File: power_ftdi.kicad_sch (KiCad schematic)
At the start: 2 parts, among them J3 USB_C_Receptacle_USB2.0_14P, U3 FT4232H

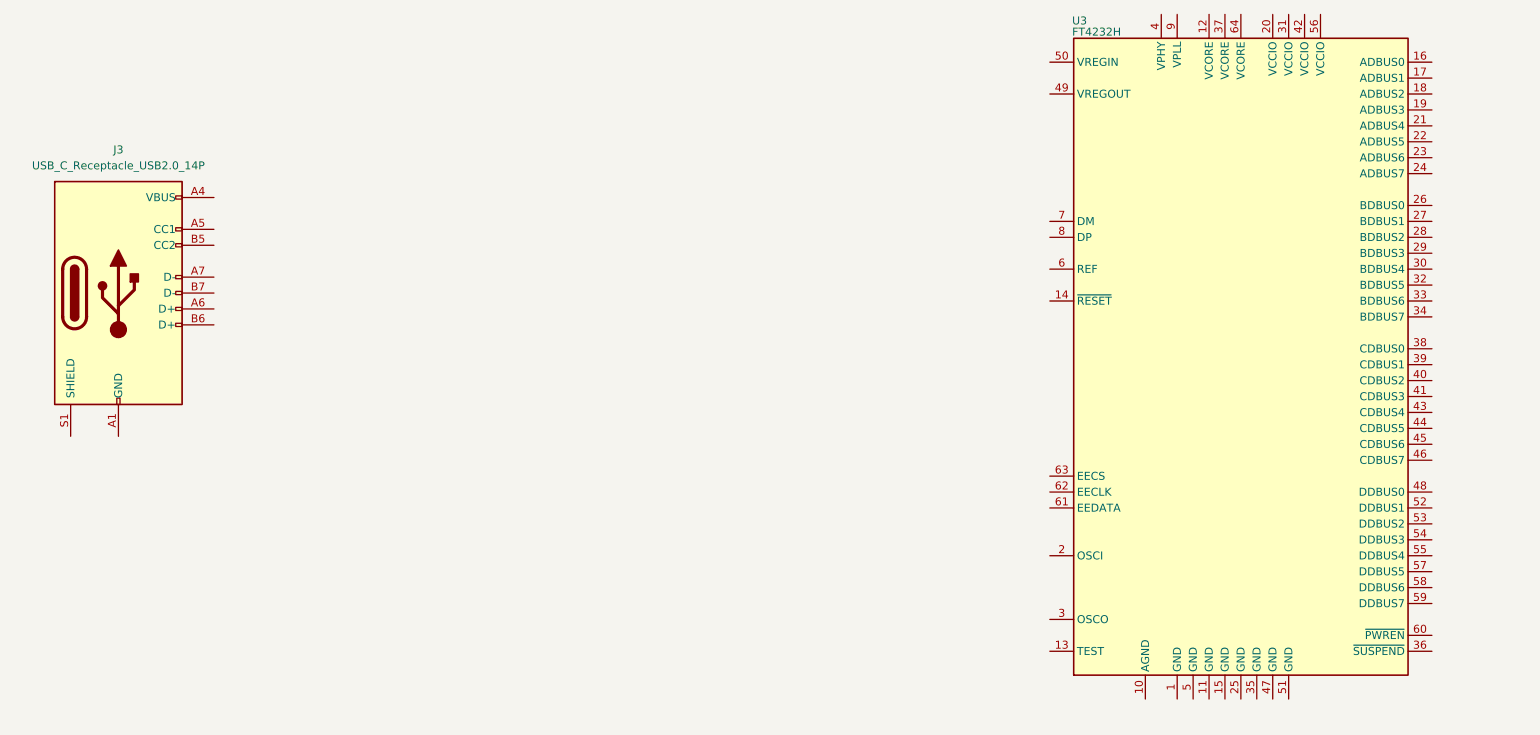
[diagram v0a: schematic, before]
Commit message: develop: Did some stuff. Not sure what I am doing :).
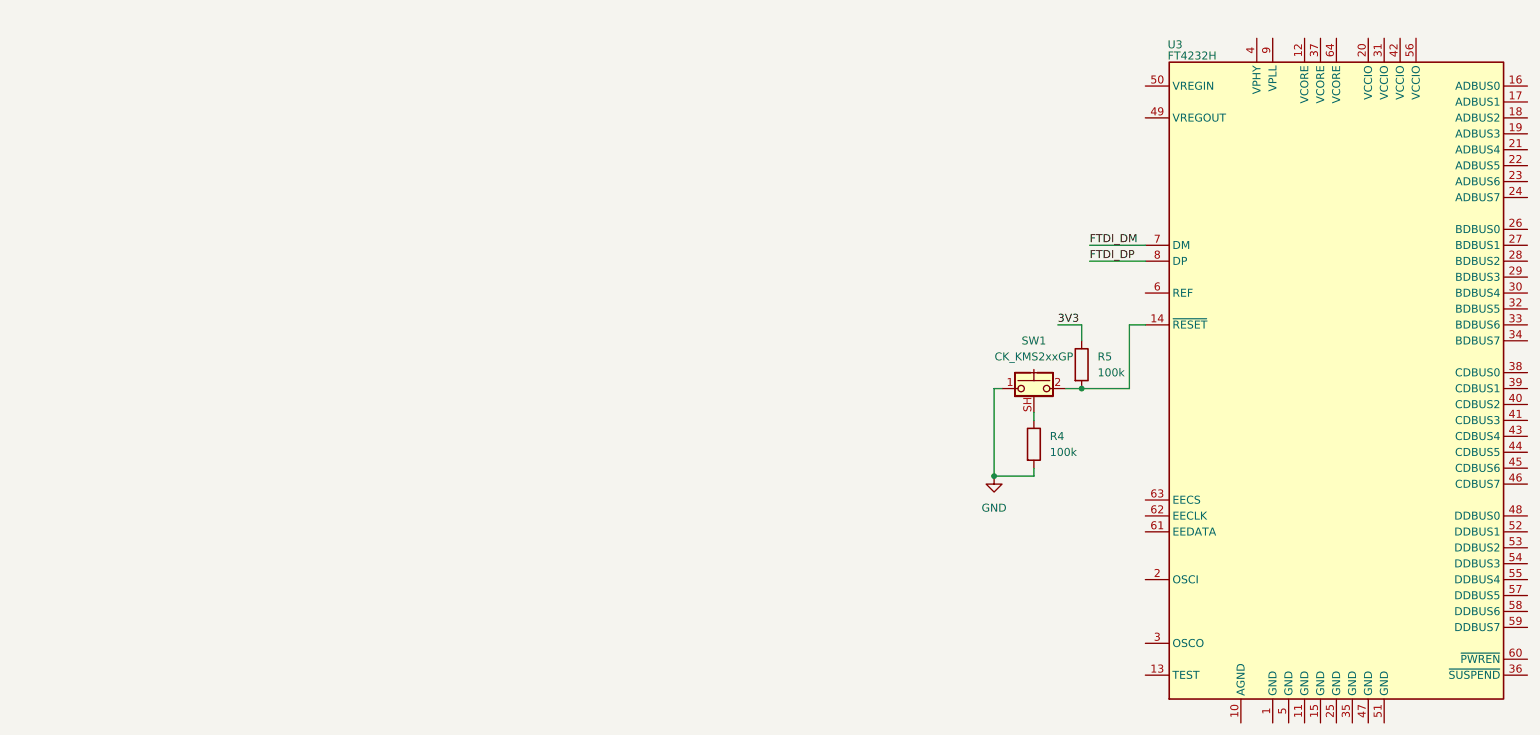
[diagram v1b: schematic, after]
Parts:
- removed J3: USB_C_Receptacle_USB2.0_14P, symbol Connector:USB_C_Receptacle_USB2.0_14P
- added R4, R5: 100k, symbol Device:R
- added SW1: CK_KMS2xxGP, Button_Switch_SMD:SW_SPST_CK_KMS2xxGP, symbol Switch:CK_KMS2xxGP
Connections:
- net at U3.14 (~{RESET}): now also R5.2, SW1.2
- net FTDI_DM: now reaches U3.7 (DM)
- net FTDI_DP: now reaches U3.8 (DP)
- new net: R4.1, SW1.SH (B)
- new net 3V3: R5.1
- new net GND: R4.2, SW1.1
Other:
- moved on the sheet: U3
